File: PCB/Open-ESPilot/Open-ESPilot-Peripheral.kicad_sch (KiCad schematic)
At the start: 57 parts, among them J10 UART1, J11 UART2, J12 I2C, J13 Micro SD Card Breakout, J14 LED out, J5 PWM output, J6 RC in, J7 Vx, J8 GND, J9 UART0, M2 GY91, Q2 BC847, Q3 BC847, U5 Micro_SD_Card

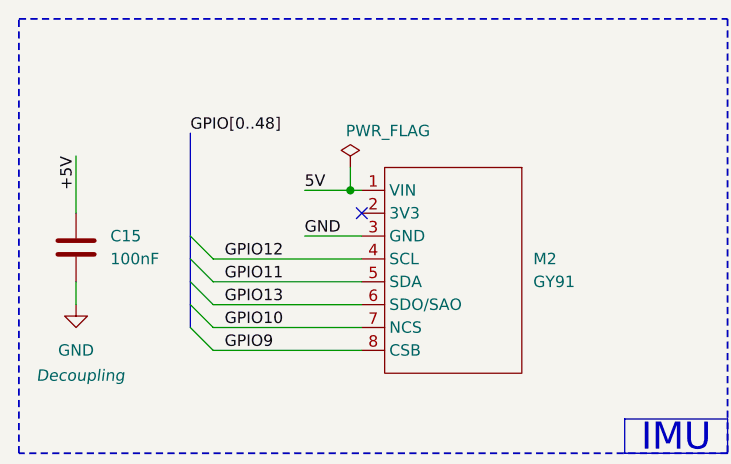
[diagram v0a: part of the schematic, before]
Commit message: PCB init.
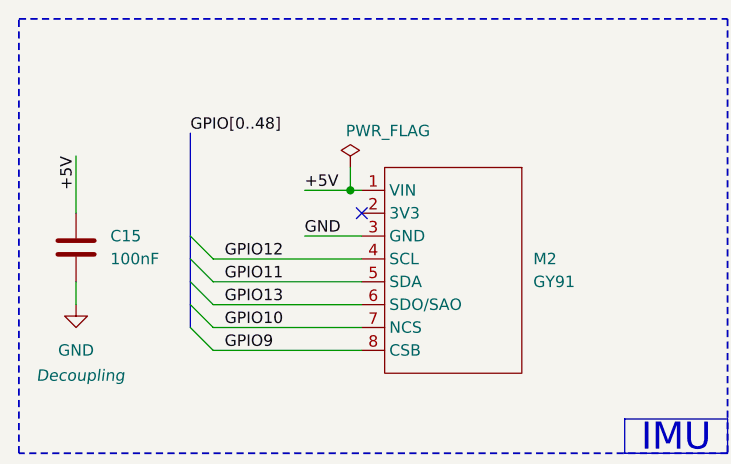
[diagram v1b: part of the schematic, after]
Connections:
- net +5V: now also M2.1 (VIN)
- net 5V: no longer M2.1 (VIN)
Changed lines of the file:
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@@
 		)
 	)
-	(label "5V"
+	(label "+5V"
 		(at 48.26 36.83 0)
 		(effects
